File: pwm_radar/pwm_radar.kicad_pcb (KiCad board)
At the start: 2 copper layers, 39 x 39 mm, 18 parts, among them J1 Conn_Coaxial, J2 Conn_01x01_Pin, J3 Conn_01x01_Pin, J4 Conn_Coaxial, J5 Conn_Coaxial, J6 Conn_Coaxial, J7 Conn_01x01_Pin, J8 Conn_01x01_Pin

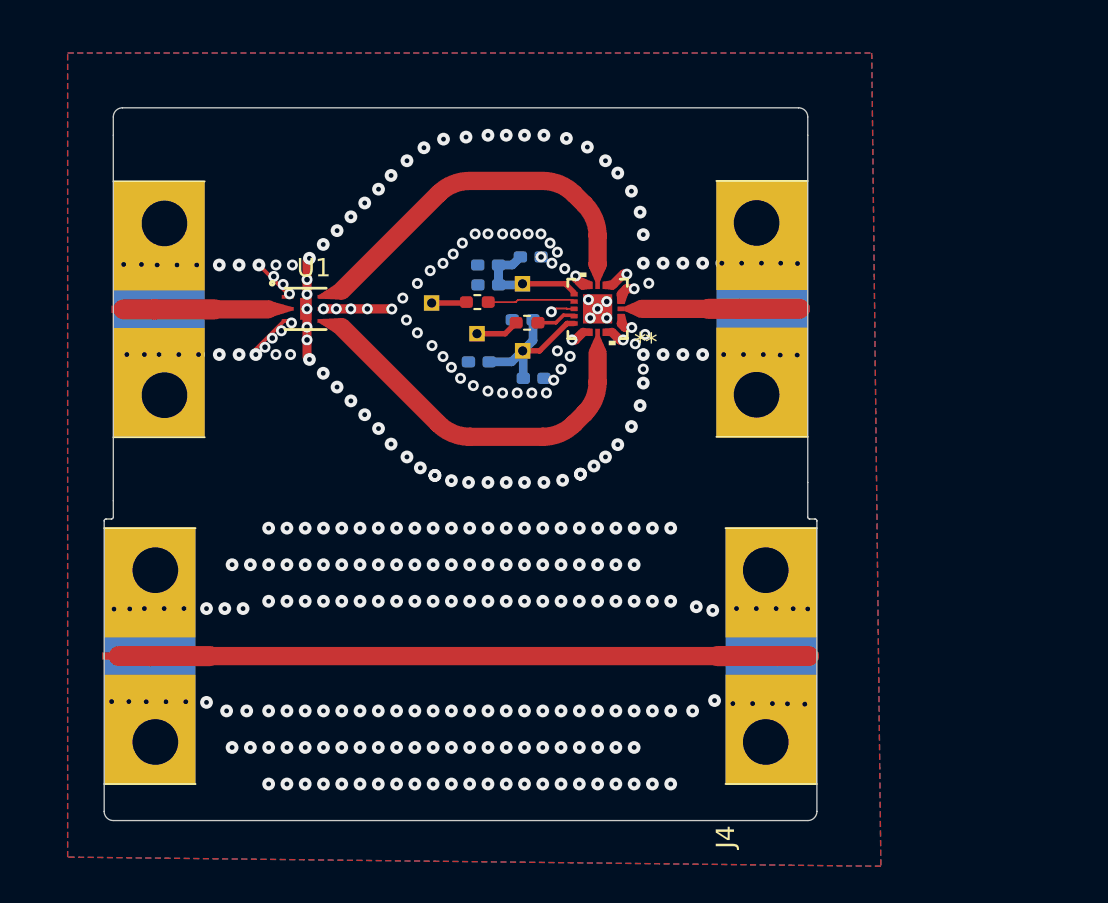
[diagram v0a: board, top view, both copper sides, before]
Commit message: updates
updates
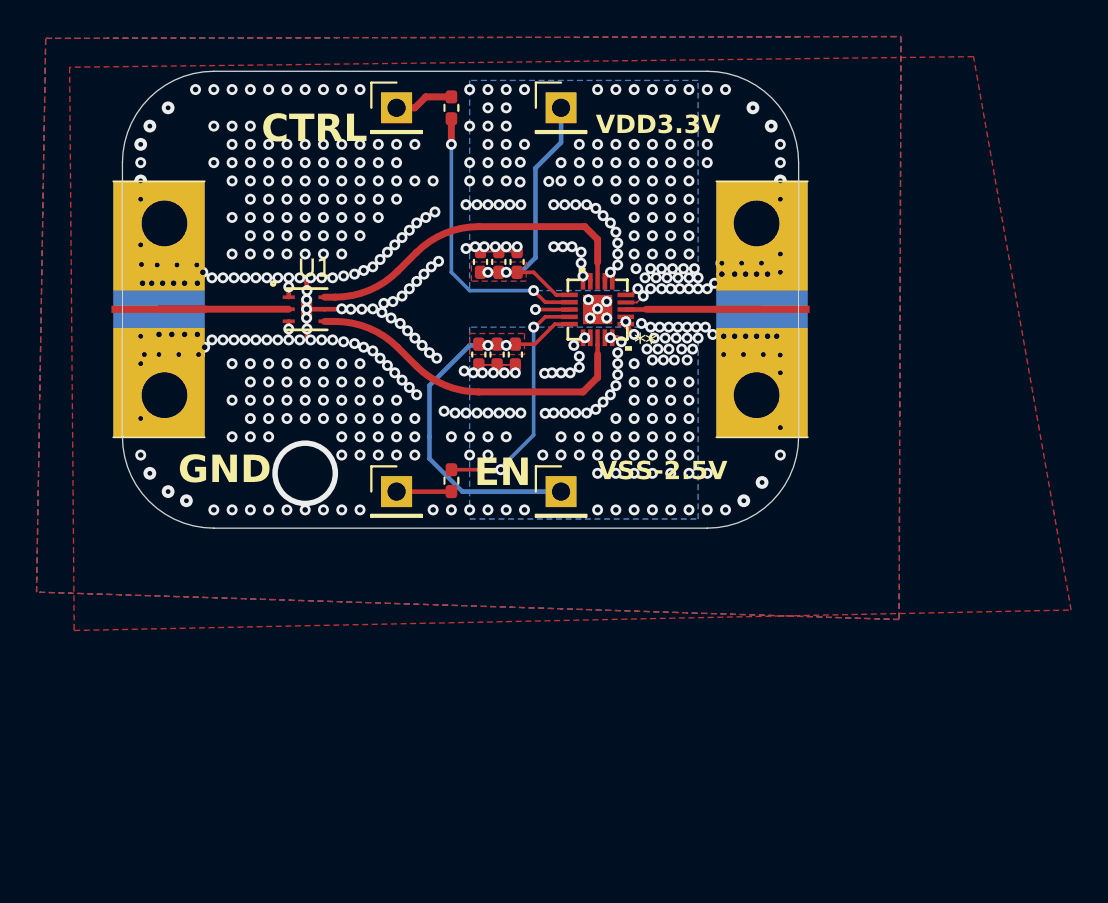
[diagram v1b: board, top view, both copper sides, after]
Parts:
- removed J4, J5: Conn_Coaxial, pwm_radar_lib:Wurth_RF_PWM_Conn
- C1, C2, C3, C4, C5, C6: moved to F.Cu
- J2, J3, J7, J8: footprint Connector_PinHeader_1.00mm:PinHeader_1x01_P1.00mm_Vertical -> Connector_PinHeader_2.54mm:PinHeader_1x01_P2.54mm_Vertical; moved to F.Cu
- moved J2 10.9 mm to (103.0, 46.0), turned to 0 degrees
- moved R1 10.7 mm to (106.0, 46.0), turned to 90 degrees
- moved J3 9.86 mm to (112.0, 46.0), turned to 0 degrees
- moved J7 9.70 mm to (103.0, 67.0), turned to 0 degrees
- moved R2 9.58 mm to (106.0, 66.4), turned to -90 degrees
- moved J8 7.98 mm to (112.0, 67.0), turned to 0 degrees
- moved C4 3.06 mm to (107.5, 59.5), turned to -90 degrees
- moved C1 2.76 mm to (107.6, 54.4), turned to 90 degrees
- moved C6 2.39 mm to (108.5, 59.5), turned to -90 degrees
- moved C5 2.04 mm to (109.5, 59.5), turned to -90 degrees
- moved C3 2.01 mm to (109.6, 54.4), turned to 90 degrees
- moved C2 0.61 mm to (108.6, 54.4), turned to 90 degrees
- moved U1 0.06 mm to (98.1, 57.0)
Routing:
- net Net-(J4-In): track 42.7 -> 0.00 mm
- net VSS: track 8.97 -> 21.5 mm, vias 0 -> 2
- net EN: track 2.15 -> 13.4 mm, vias 0 -> 2
- net CTRL: track 4.90 -> 15.5 mm, vias 0 -> 2
- net VDD: track 6.82 -> 17.2 mm, vias 0 -> 2
- net Net-(J6-In): track 13.6 -> 7.46 mm
- net Net-(J1-In): track 12.9 -> 7.10 mm
- net GND: track 20.3 -> 25.3 mm, vias 320 -> 525
- net RF1+: track 19.5 -> 17.6 mm
- net RF1-: track 19.5 -> 17.7 mm
- net Net-(J2-Pin_1): track 1.92 -> 3.25 mm
- net Net-(J7-Pin_1): track 2.39 -> 3.00 mm
- added copper zone on In1.Cu, net GND
- added copper zone on In2.Cu, net GND
- added copper zone on B.Cu, net VDD
- added copper zone on F.Cu, net VDD
- added copper zone on B.Cu, net VSS
- added copper zone on F.Cu, net VSS
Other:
- board size 39 x 39 mm -> 37 x 25 mm
- copper layers 2 -> 4
- board text added: "CTRL"
- board text added: "EN"
- board text added: "GND"
- board text added: "VDD3.3V"
- board text added: "VSS-2.5V"
